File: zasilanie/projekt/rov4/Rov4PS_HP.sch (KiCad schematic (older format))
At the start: 71 parts, among them IC2 UWE-12_10-Q12PB-C, J23 HP_Enable, J24 Manip_sil_12v, J25 Torp_EleMagnes, J26 Extra, J27 RC_HP_12V, J28 Extra, J29 Torpedy_serwo_7v, J30 Extra, J31 Extra, J32 Manip_serwo, J33 Extra, J34 Extra, J35 Manip_Silnik_1, J36 Manip_Silnik_2, J37 Extra, J38 Extra, J39 ESC1, J40 ESC2, J41 ESC3, J42 ESC4, J43 ESC5, J44 ESC6, J45 ESC7, J46 ESC8, Q6 IPT004N03L, Q7 IPT004N03L, Q8 IPT004N03L, Q9 IPT004N03L, U2 Transoptor, U3 Transoptor, U4 lm2596, U5 lm2596, U6 XL4015

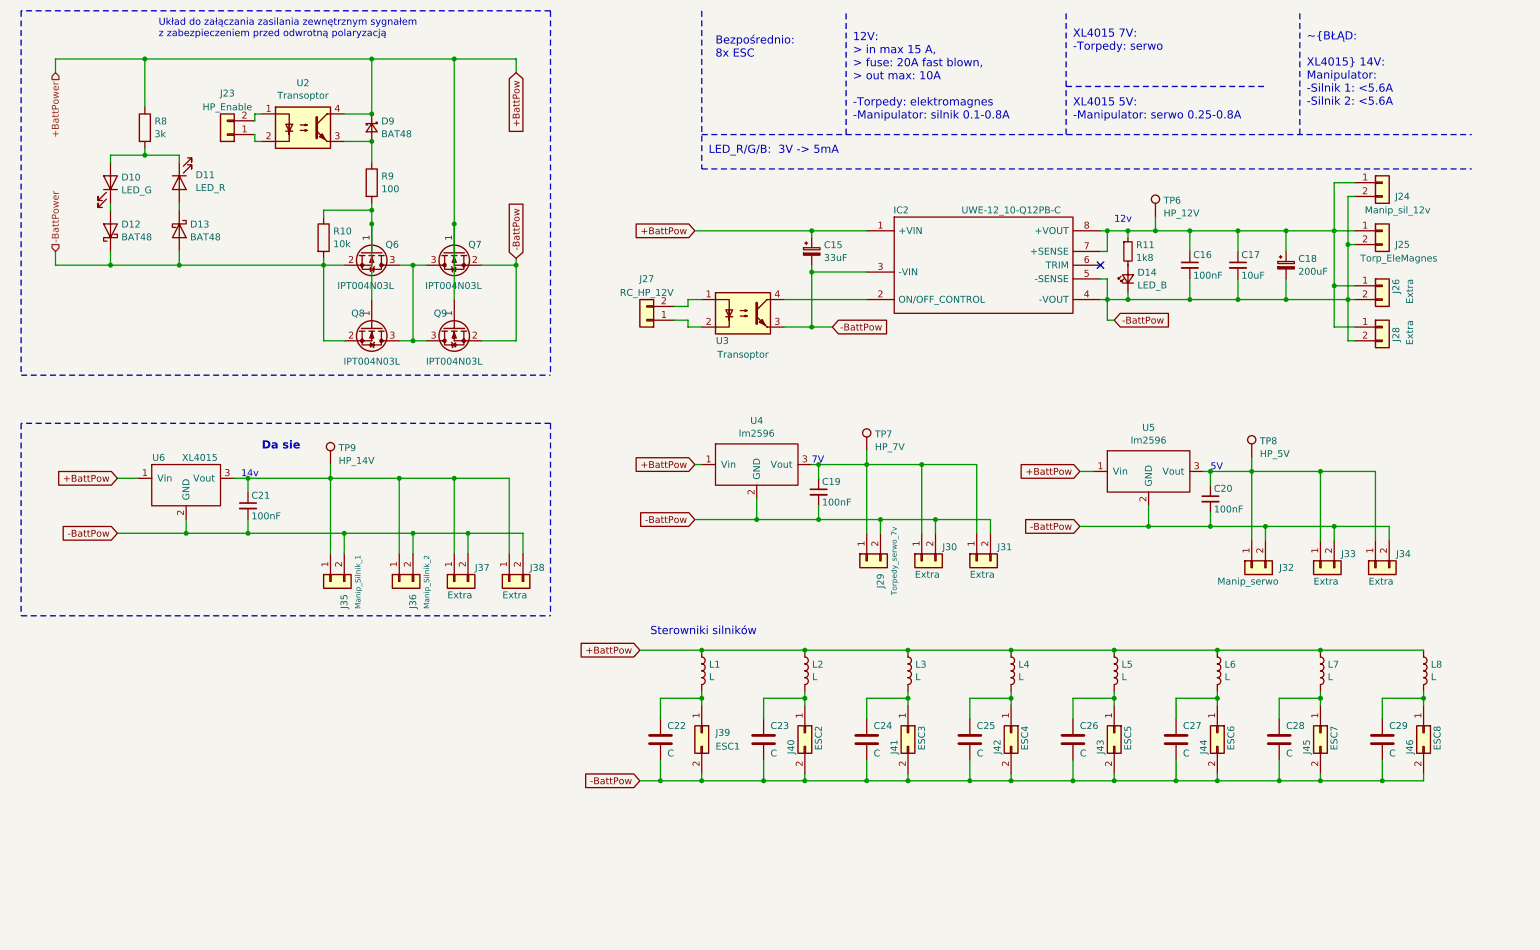
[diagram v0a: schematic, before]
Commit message: sync
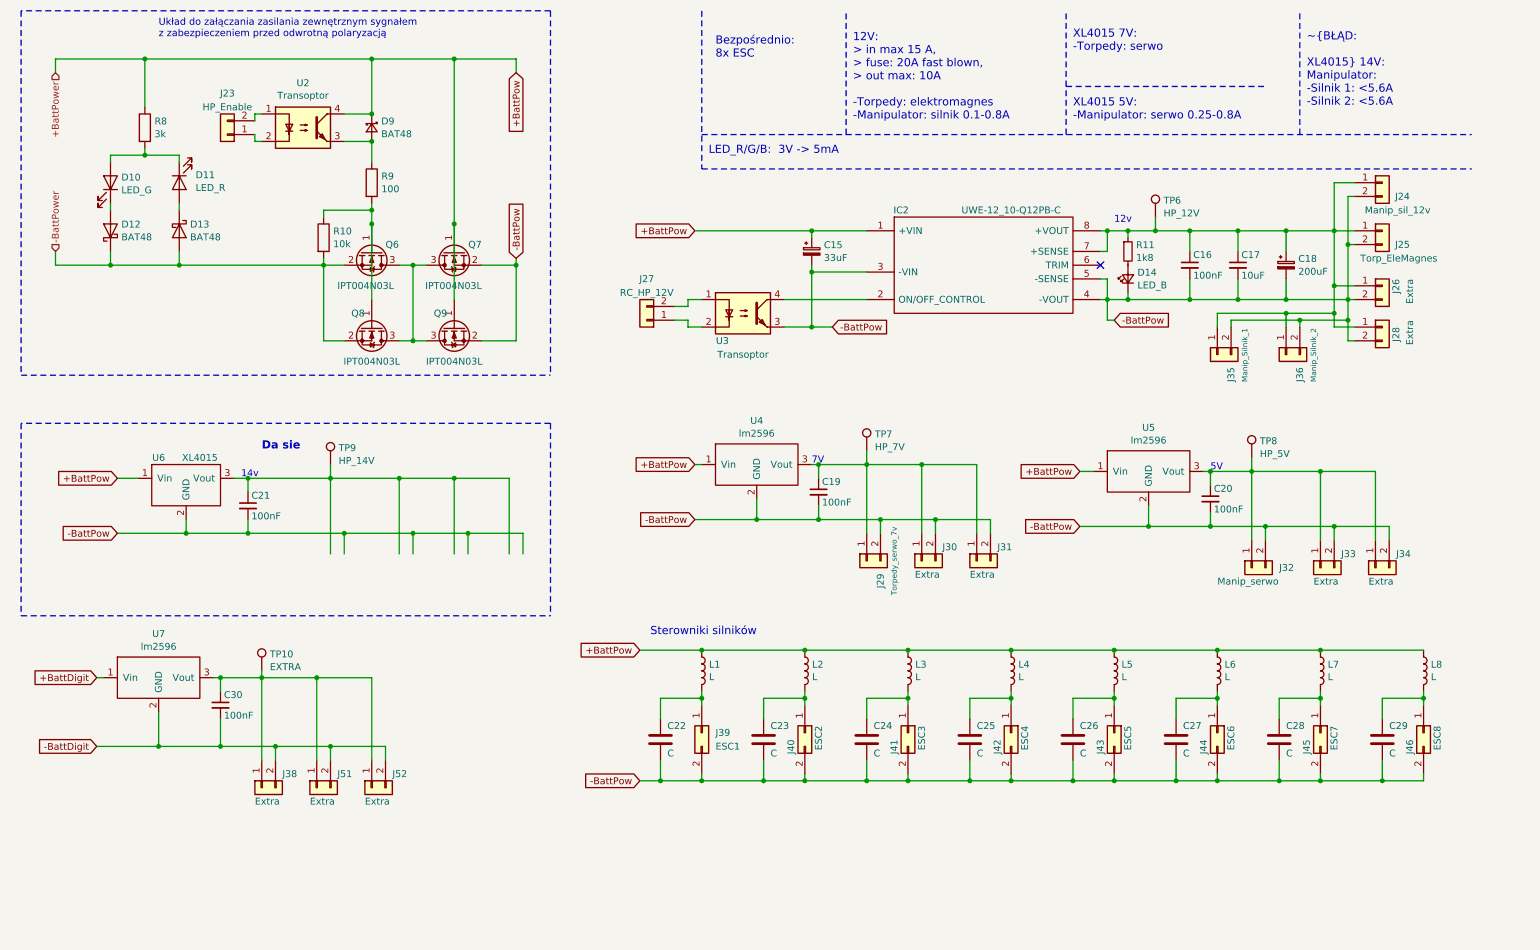
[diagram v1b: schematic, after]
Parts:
- removed J37: Extra, Connector_PinHeader_2.54mm:PinHeader_1x02_P2.54mm_Vertical, symbol Connector_Generic:Conn_01x02
- added C30: 100nF, Capacitor_SMD:C_0805_2012Metric, symbol Device:C_Small
- added J51, J52: Extra, Connector_PinHeader_2.54mm:PinHeader_1x02_P2.54mm_Vertical, symbol Connector_Generic:Conn_01x02
- added TP10: EXTRA, Connector_PinHeader_2.54mm:PinHeader_1x01_P2.54mm_Vertical, symbol Connector:TestPoint
- added U7: lm2596, lm2596:lm2596-44_8mm_x_23mm, symbol lm2596:lm2596
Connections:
- net labels added: +BattDigit, -BattDigit
- wire segments 241 -> 271
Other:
- moved on the sheet: J35, J36
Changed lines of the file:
@@
 L Connector_Generic:Conn_01x02 J?
 U 1 1 5C9B947B
-P 2850 4700
+P 9300 3050
 AR Path="/5C9B947B" Ref="J?"  Part="1"
 AR Path="/5C93D53B/5C9B947B" Ref="J35"  Part="1"
-F 0 "J35" H 3050 4600 50  0000 R CNN
-F 1 "Manip_Silnik_1" H 3050 4500 39  0000 R CNN
-F 2 "Connector_PinHeader_2.54mm:PinHeader_1x02_P2.54mm_Vertical" H 2850 4700 50  0001 C CNN
-F 3 "~" H 2850 4700 50  0001 C CNN
-	1    2850 4700
+F 0 "J35" H 9500 2950 50  0000 R CNN
+F 1 "Manip_Silnik_1" H 9500 2850 39  0000 R CNN
+F 2 "Connector_PinHeader_2.54mm:PinHeader_1x02_P2.54mm_Vertical" H 9300 3050 50  0001 C CNN
+F 3 "~" H 9300 3050 50  0001 C CNN
+	1    9300 3050
 	0    -1   1    0
 $EndComp
@@
 L Connector_Generic:Conn_01x02 J?
 U 1 1 5C9C12E4
-P 3350 4700
+P 9800 3050
 AR Path="/5C9C12E4" Ref="J?"  Part="1"
 AR Path="/5C93D53B/5C9C12E4" Ref="J36"  Part="1"
-F 0 "J36" H 3550 4600 50  0000 R CNN
-F 1 "Manip_Silnik_2" H 3550 4500 39  0000 R CNN
-F 2 "Connector_PinHeader_2.54mm:PinHeader_1x02_P2.54mm_Vertical" H 3350 4700 50  0001 C CNN
-F 3 "~" H 3350 4700 50  0001 C CNN
-	1    3350 4700
+F 0 "J36" H 10000 2950 50  0000 R CNN
+F 1 "Manip_Silnik_2" H 10000 2850 39  0000 R CNN
+F 2 "Connector_PinHeader_2.54mm:PinHeader_1x02_P2.54mm_Vertical" H 9800 3050 50  0001 C CNN
+F 3 "~" H 9800 3050 50  0001 C CNN
+	1    9800 3050
 	0    -1   1    0
 $EndComp
@@
 	1    10500 2850
 	1    0    0    -1
-$EndComp
-$Comp
-L Connector_Generic:Conn_01x02 J?
-U 1 1 5CAF206E
-P 4150 4700
-AR Path="/5CAF206E" Ref="J?"  Part="1"
-AR Path="/5C93D53B/5CAF206E" Ref="J38"  Part="1"
-F 0 "J38" V 4050 4550 50  0000 R CNN
-F 1 "Extra" V 4250 4750 50  0000 R CNN
-F 2 "Connector_PinHeader_2.54mm:PinHeader_1x02_P2.54mm_Vertical" H 4150 4700 50  0001 C CNN
-F 3 "~" H 4150 4700 50  0001 C CNN
-	1    4150 4700
-	0    -1   1    0
-$EndComp
-$Comp
-L Connector_Generic:Conn_01x02 J?
-U 1 1 5CAF2075
-P 3750 4700
-AR Path="/5CAF2075" Ref="J?"  Part="1"
-AR Path="/5C93D53B/5CAF2075" Ref="J37"  Part="1"
-F 0 "J37" V 3650 4550 50  0000 R CNN
-F 1 "Extra" V 3850 4750 50  0000 R CNN
-F 2 "Connector_PinHeader_2.54mm:PinHeader_1x02_P2.54mm_Vertical" H 3750 4700 50  0001 C CNN
-F 3 "~" H 3750 4700 50  0001 C CNN
-	1    3750 4700
-	0    -1   1    0
 $EndComp
 $Comp
@@
 Connection ~ 10150 2550
 Wire Wire Line
-	10150 2550 10150 2850
+	10150 2550 10150 2750
 Wire Wire Line
 	10300 2850 10150 2850
@@
 	10300 2950 10250 2950
 Wire Wire Line
-	10250 2950 10250 2650
+	10250 2950 10250 2800
 Connection ~ 10250 2250
 Connection ~ 10250 2650
@@
 	9200 3900 9250 3900
 Connection ~ 9250 3900
+$Comp
+L Connector_Generic:Conn_01x02 J52
+U 1 1 5CC73B50
+P 3150 6200
+F 0 "J52" V 3050 6050 50  0000 R CNN
+F 1 "Extra" V 3250 6250 50  0000 R CNN
+F 2 "Connector_PinHeader_2.54mm:PinHeader_1x02_P2.54mm_Vertical" H 3150 6200 50  0001 C CNN
+F 3 "~" H 3150 6200 50  0001 C CNN
+	1    3150 6200
+	0    -1   1    0
+$EndComp
+$Comp
+L Connector_Generic:Conn_01x02 J51
+U 1 1 5CC73B57
+P 2750 6200
+F 0 "J51" V 2650 6050 50  0000 R CNN
+F 1 "Extra" V 2850 6250 50  0000 R CNN
+F 2 "Connector_PinHeader_2.54mm:PinHeader_1x02_P2.54mm_Vertical" H 2750 6200 50  0001 C CNN
+F 3 "~" H 2750 6200 50  0001 C CNN
+	1    2750 6200
+	0    -1   1    0
+$EndComp
+$Comp
+L Connector_Generic:Conn_01x02 J38
+U 1 1 5CC73B5E
+P 2350 6200
+F 0 "J38" V 2250 6050 50  0000 R CNN
+F 1 "Extra" V 2450 6250 50  0000 R CNN
+F 2 "Connector_PinHeader_2.54mm:PinHeader_1x02_P2.54mm_Vertical" H 2350 6200 50  0001 C CNN
+F 3 "~" H 2350 6200 50  0001 C CNN
+	1    2350 6200
+	0    -1   1    0
+$EndComp
+Wire Wire Line
+	2350 5400 2350 6000
+Wire Wire Line
+	2450 5900 2850 5900
+Wire Wire Line
+	3250 6000 3250 5900
+Wire Wire Line
+	2850 6000 2850 5900
+Connection ~ 2850 5900
+Wire Wire Line
+	2850 5900 3250 5900
+Wire Wire Line
+	2750 6000 2750 5400
+Connection ~ 2750 5400
+Wire Wire Line
+	2750 5400 2350 5400
+Wire Wire Line
+	3150 6000 3150 5400
+Wire Wire Line
+	2750 5400 3150 5400
+Connection ~ 2450 5900
+Wire Wire Line
+	2450 5900 2450 6000
+Connection ~ 2350 5400
+Text GLabel 1150 5400 0    50   Input ~ 0
++BattDigit
+$Comp
+L Connector:TestPoint TP10
+U 1 1 5CC73B74
+P 2350 5350
+F 0 "TP10" H 2409 5471 50  0000 L CNN
+F 1 "EXTRA" H 2409 5378 50  0000 L CNN
+F 2 "Connector_PinHeader_2.54mm:PinHeader_1x01_P2.54mm_Vertical" H 2550 5350 50  0001 C CNN
+F 3 "~" H 2550 5350 50  0001 C CNN
+	1    2350 5350
+	1    0    0    -1
+$EndComp
+Wire Wire Line
+	2350 5400 2350 5350
+$Comp
+L Device:C_Small C?
+U 1 1 5CC73B7C
+P 2050 5600
+AR Path="/5CC73B7C" Ref="C?"  Part="1"
+AR Path="/5C93D53B/5CC73B7C" Ref="C30"  Part="1"
+F 0 "C30" H 2075 5675 50  0000 L CNN
+F 1 "100nF" H 2075 5525 50  0000 L CNN
+F 2 "Capacitor_SMD:C_0805_2012Metric" H 2050 5600 50  0001 C CNN
+F 3 "~" H 2050 5600 50  0001 C CNN
+	1    2050 5600
+	1    0    0    -1
+$EndComp
+Wire Wire Line
+	2050 5500 2050 5400
+Wire Wire Line
+	2050 5700 2050 5900
+Connection ~ 2050 5900
+Wire Wire Line
+	2050 5900 2450 5900
+Wire Wire Line
+	2000 5400 2050 5400
+Wire Wire Line
+	2350 5400 2050 5400
+Connection ~ 2050 5400
+Text GLabel 1150 5900 0    50   Input ~ 0
+-BattDigit
+$Comp
+L lm2596:lm2596 U7
+U 1 1 5CC73B8B
+P 1600 5400
+F 0 "U7" H 1600 5719 50  0000 C CNN
+F 1 "lm2596" H 1600 5626 50  0000 C CNN
+F 2 "lm2596:lm2596-44_8mm_x_23mm" H 1600 5300 50  0001 C CNN
+F 3 "" H 1600 5300 50  0001 C CNN
+	1    1600 5400
+	1    0    0    -1
+$EndComp
+Wire Wire Line
+	1600 5650 1600 5900
+Wire Wire Line
+	1600 5900 2050 5900
+Connection ~ 1600 5900
+Wire Wire Line
+	1200 5400 1150 5400
+Wire Wire Line
+	1150 5900 1600 5900
+Wire Wire Line
+	9300 2850 9300 2750
+Wire Wire Line
+	9300 2750 9800 2750
+Connection ~ 10150 2750
+Wire Wire Line
+	10150 2750 10150 2850
+Wire Wire Line
+	9800 2850 9800 2750
+Connection ~ 9800 2750
+Wire Wire Line
+	9800 2750 10150 2750
+Wire Wire Line
+	9400 2850 9400 2800
+Wire Wire Line
+	9400 2800 9900 2800
+Wire Wire Line
+	9900 2800 9900 2850
+Wire Wire Line
+	9900 2800 10250 2800
+Connection ~ 9900 2800
+Connection ~ 10250 2800
+Wire Wire Line
+	10250 2800 10250 2650
 $EndSCHEMATC

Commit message: test2
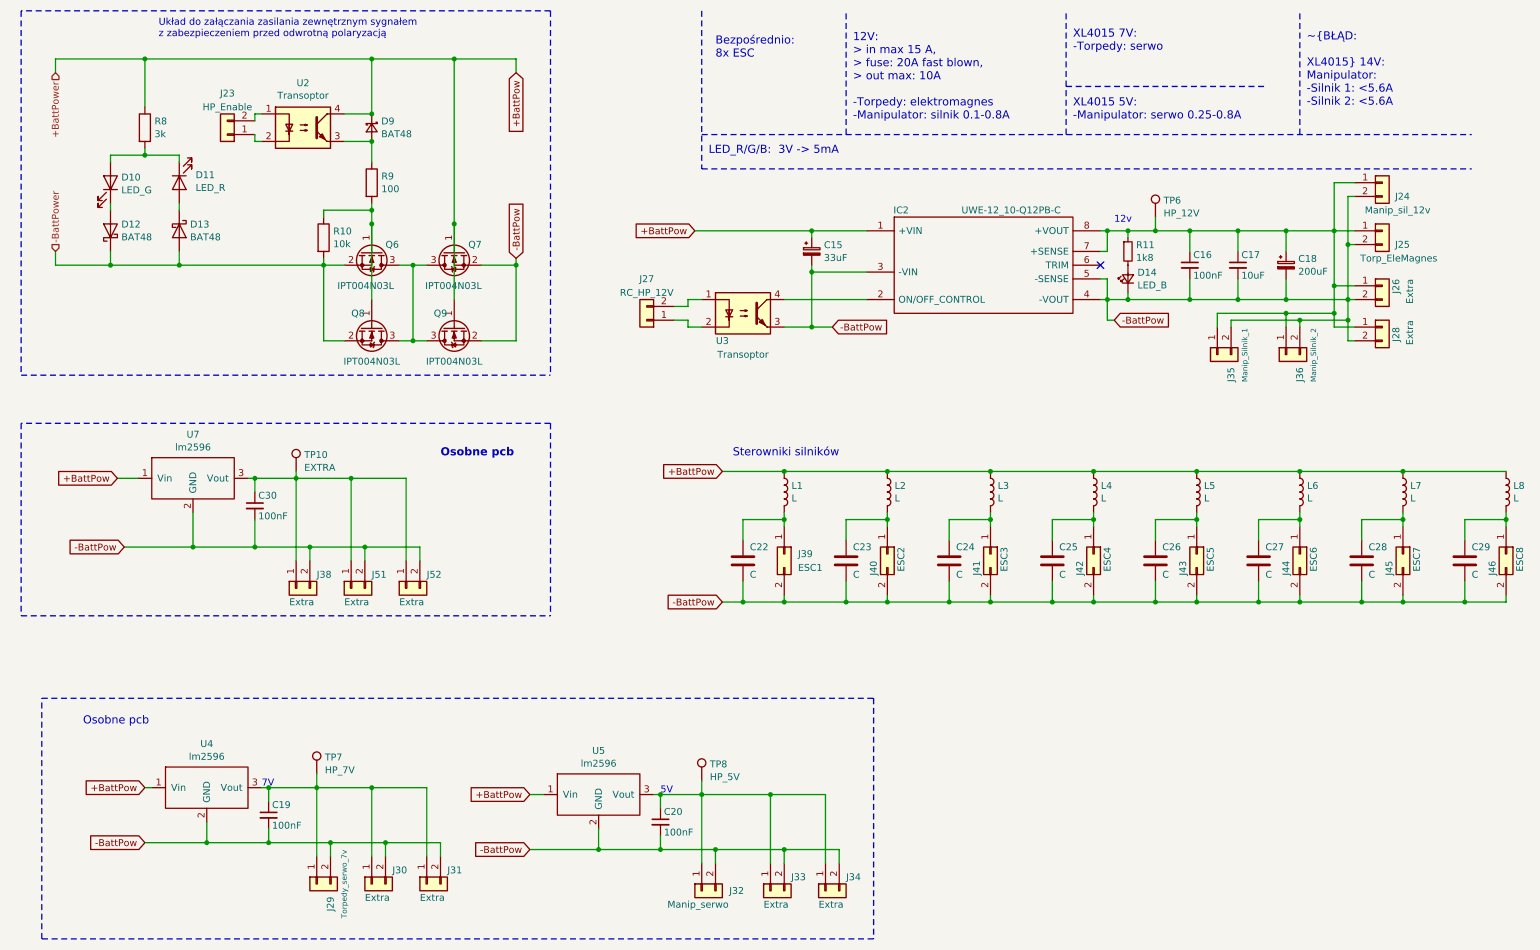
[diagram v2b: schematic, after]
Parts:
- removed C21: 100nF, Capacitor_SMD:C_0805_2012Metric, symbol Device:C_Small
- removed TP9: HP_14V, Connector_PinHeader_2.54mm:PinHeader_1x01_P2.54mm_Vertical, symbol Connector:TestPoint
- removed U6: XL4015, XL4015:xl4015, symbol XL4015:XL4015
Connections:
- net labels removed: +BattDigit, -BattDigit
- wire segments 271 -> 247
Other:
- note added: "Osobne pcb"
- note removed: "14v"
- note removed: "Da sie\n"
- moved on the sheet: C19, C20, C22, C23, C24, C25, C26, C27, C28, C29, C30, J29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
